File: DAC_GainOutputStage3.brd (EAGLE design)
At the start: 110 x 96.8 mm, 69 parts, among them J1 1935190, J3 SJ-63033A, U1 V_REG_317SMD, U2 V_REG_317SMD

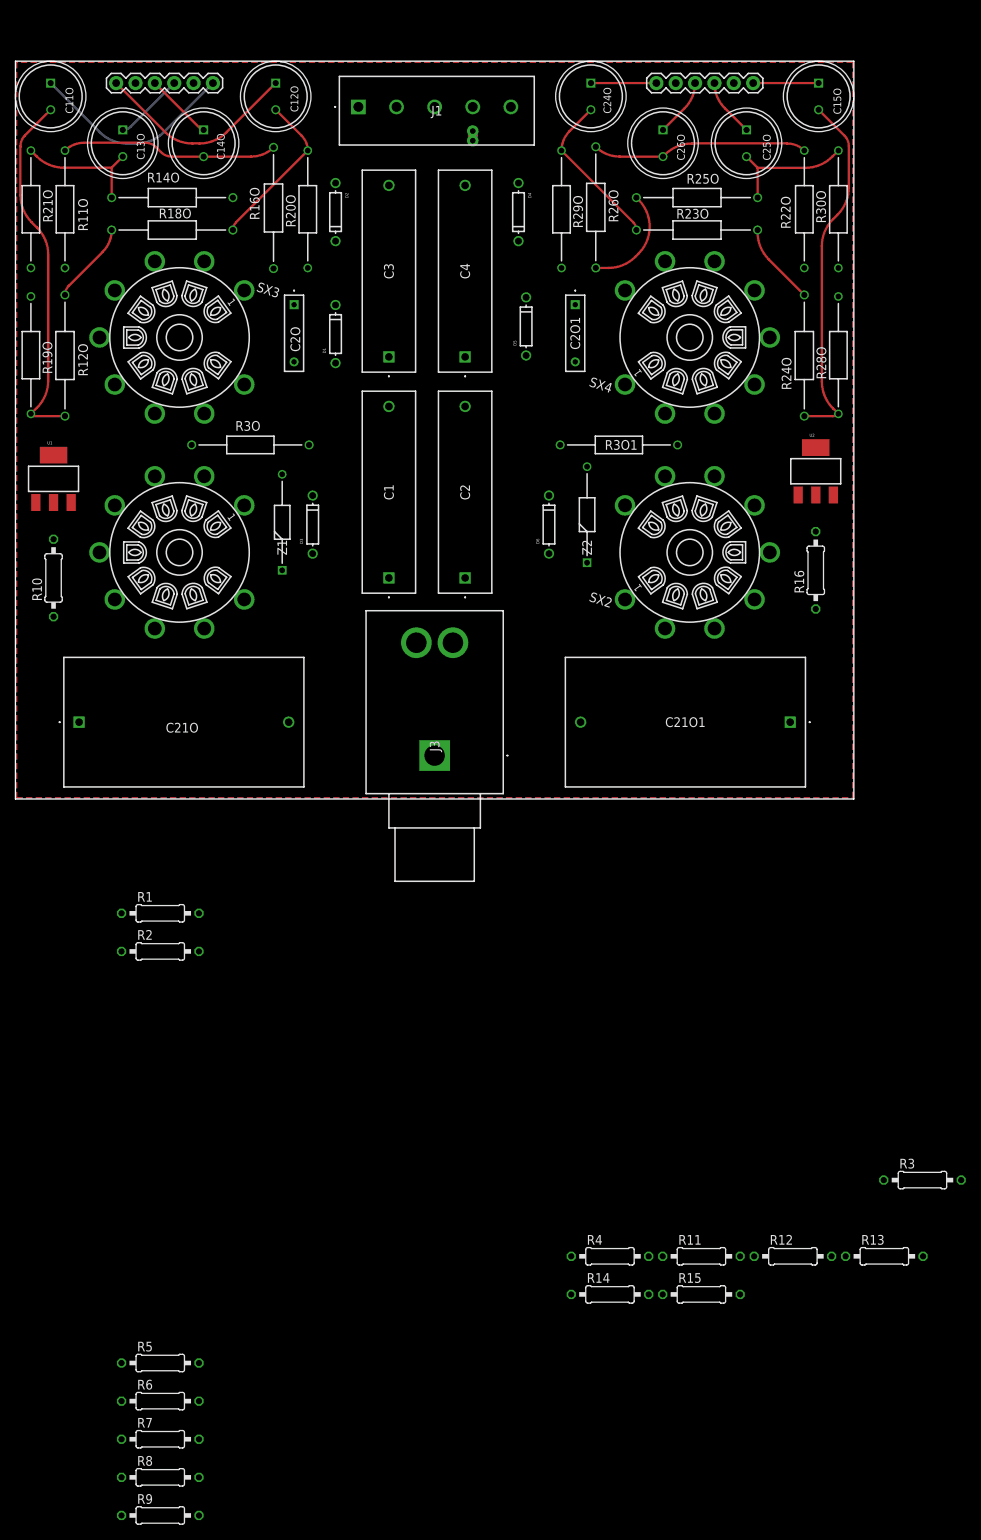
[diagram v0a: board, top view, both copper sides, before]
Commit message: Progress
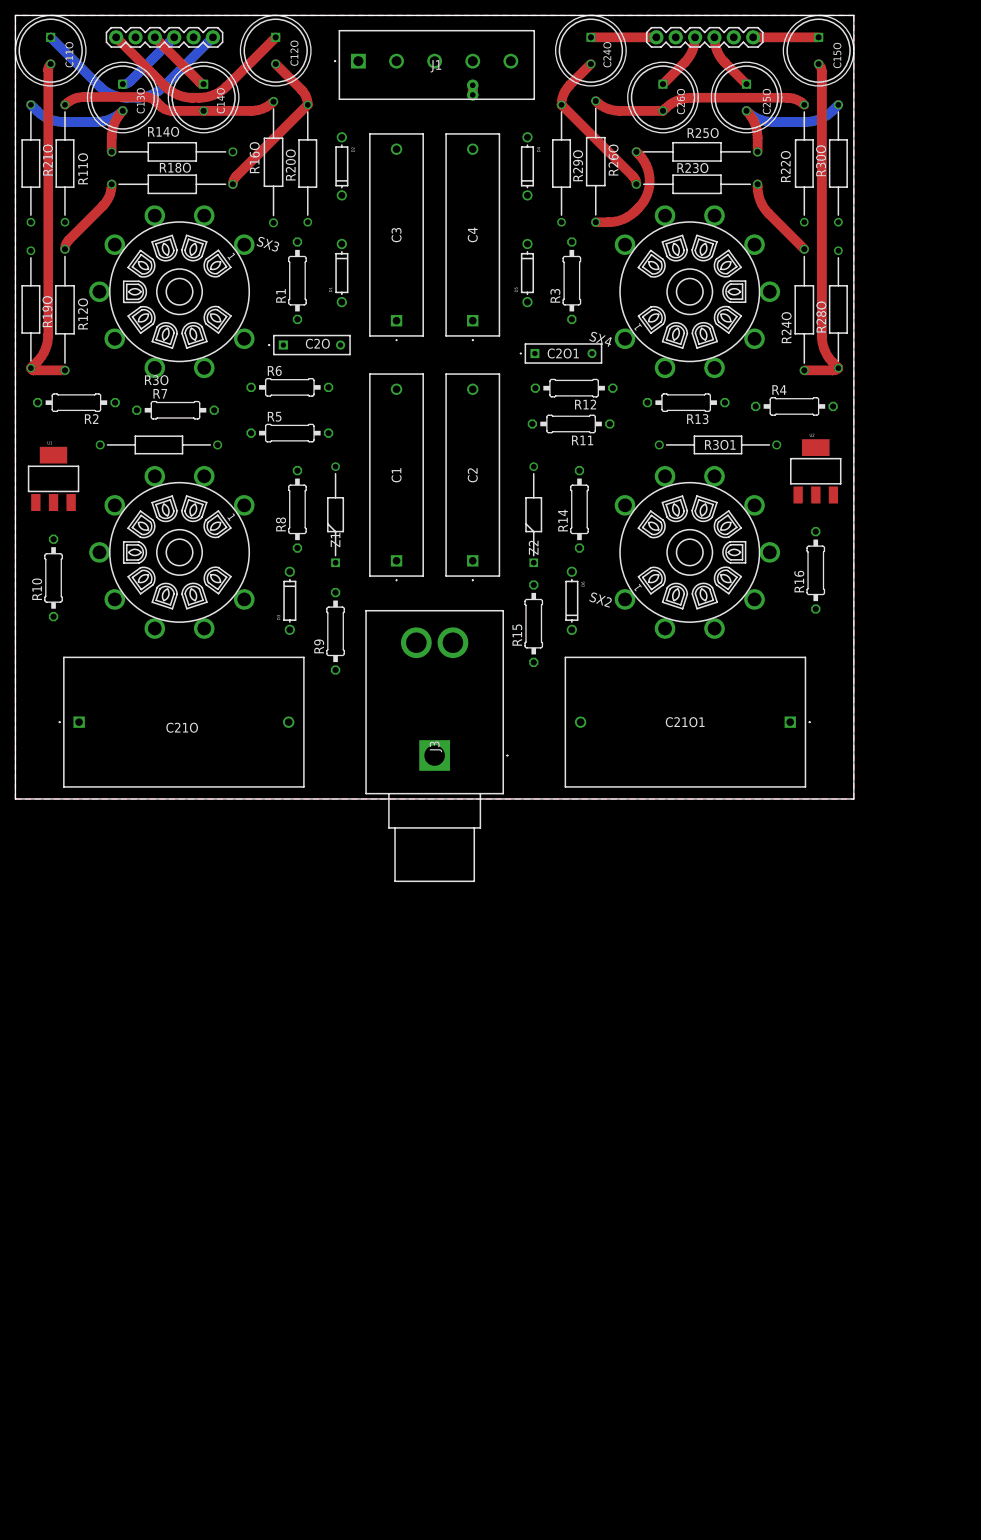
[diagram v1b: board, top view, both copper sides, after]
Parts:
- moved R7 135.0 mm to (21.0, 51.0)
- moved R6 134.1 mm to (36.0, 54.0)
- moved R8 128.3 mm to (37.0, 38.0), turned to 90 degrees
- moved R3 126.6 mm to (73.0, 68.0), turned to 90 degrees
- moved R5 123.2 mm to (36.0, 48.0)
- moved R9 118.3 mm to (42.0, 22.0), turned to 90 degrees
- moved R12 117.5 mm to (73.3, 53.9), turned to 180 degrees
- moved R13 115.0 mm to (88.0, 52.0), turned to 180 degrees
- moved R4 114.1 mm to (102.2, 51.5)
- moved R11 110.5 mm to (72.9, 49.2), turned to 180 degrees
- moved R14 103.1 mm to (74.0, 38.0), turned to 90 degrees
- moved R15 90.7 mm to (68.0, 23.0), turned to 90 degrees
- moved R1 84.9 mm to (37.0, 68.0), turned to 90 degrees
- moved R2 72.8 mm to (8.00, 52.0), turned to 180 degrees
- moved R3O1 13.0 mm to (84.5, 46.5)
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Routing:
- net N$11: track 47.5 -> 45.2 mm
- net N$20: track 47.4 -> 45.1 mm
- net N$28: track 17.2 -> 18.6 mm
- net N$36: track 17.2 -> 18.6 mm
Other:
- board size 110 x 96.8 mm -> 110 x 102.8 mm
